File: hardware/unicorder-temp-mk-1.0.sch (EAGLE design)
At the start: 13 parts, among them IC1 TINY85

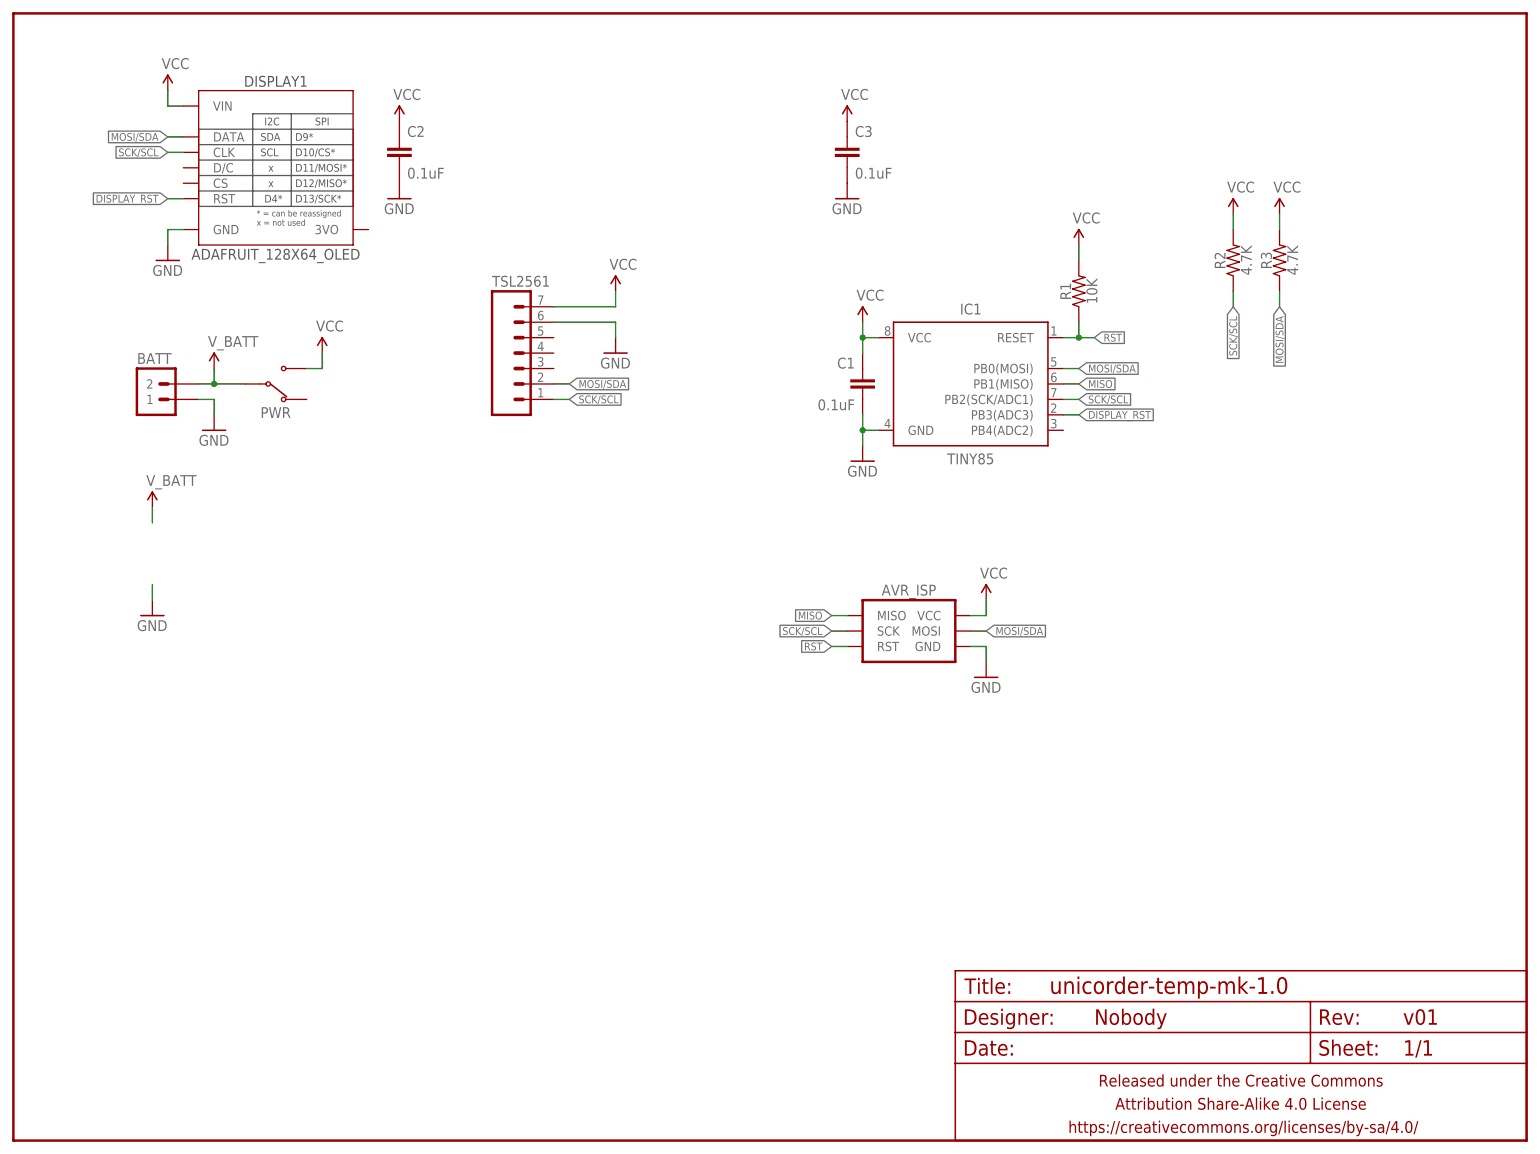
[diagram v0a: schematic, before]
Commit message: alsdkfjkalsdf
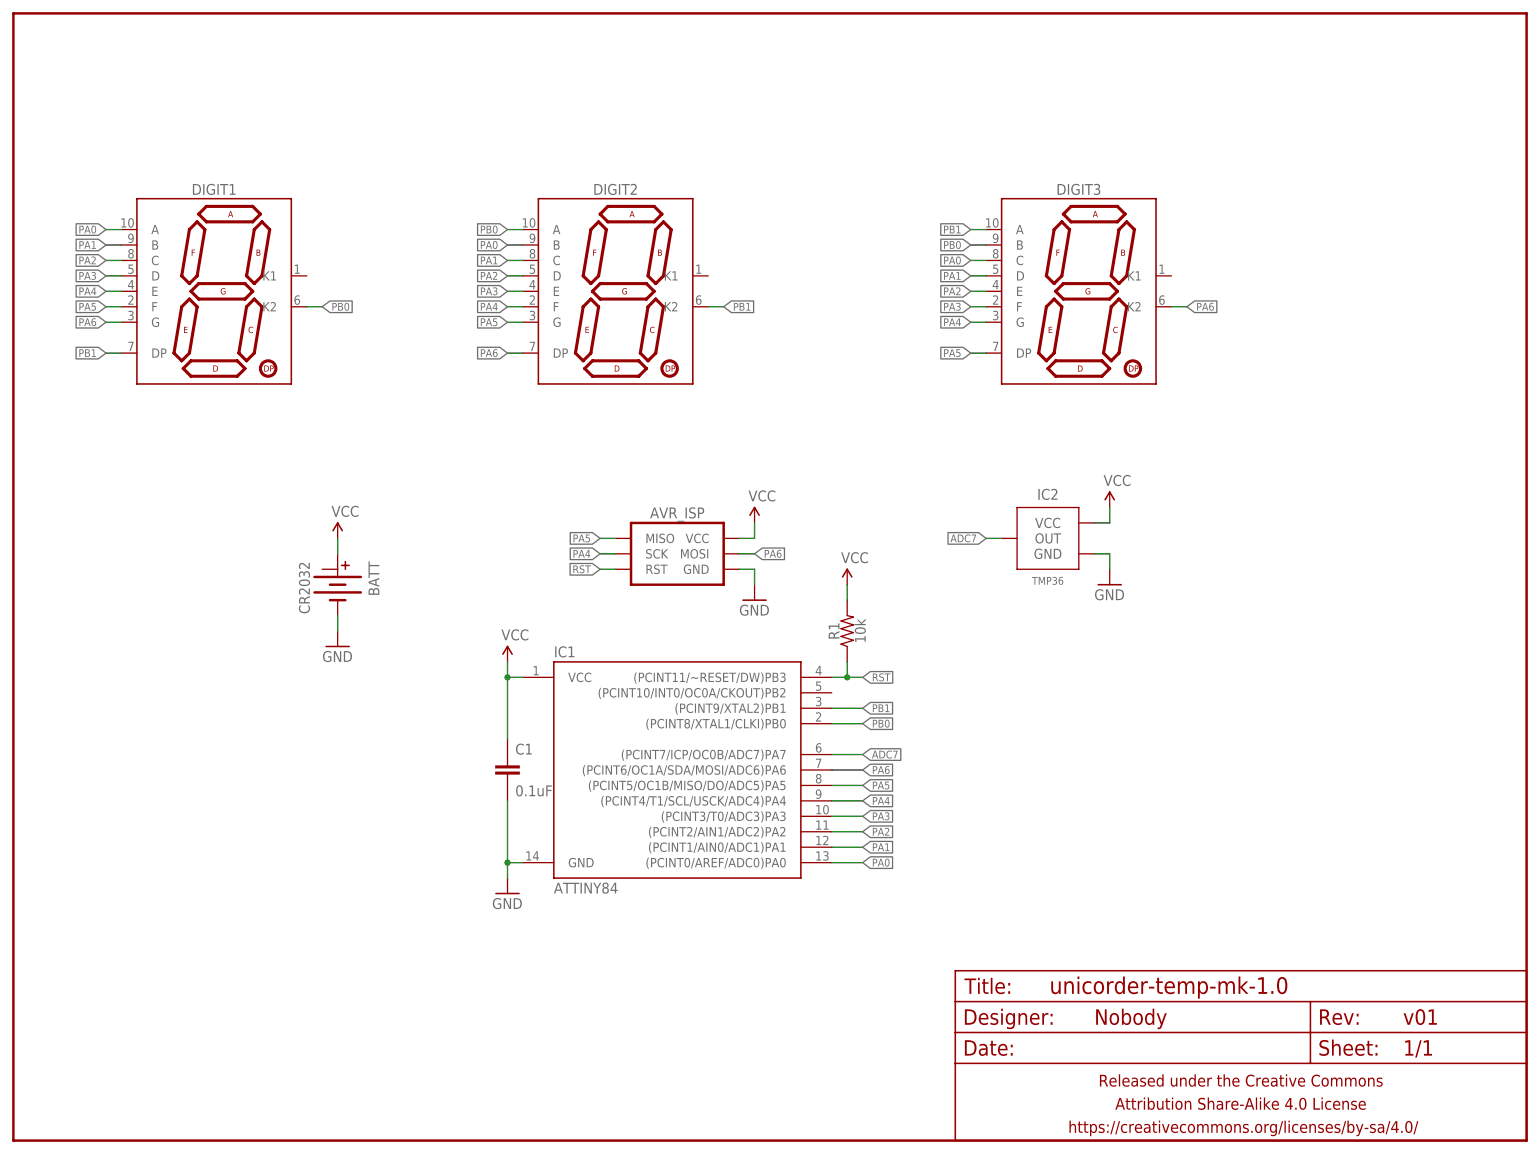
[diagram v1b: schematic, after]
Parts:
- removed C2, C3: 0.1uF, A_butts:CAPACITOR-CERAMIC025-024X044
- removed DISPLAY1: ADAFRUIT_128X64_OLED, A_butts:ADAFRUIT_128X64_OLED
- removed PWR: SWITCH-SPDTPTH-RA-2MM, A_butts:SWITCH-SPDTPTH-RA-2MM
- removed R2, R3: 4.7K, A_butts:RESISTORPTH-AXIAL-7.62MM
- removed TSL2561: (no value), A_butts:M07PTH-SLIMASS
- added DIGIT1, DIGIT2, DIGIT3: 7SEG_1DIGPTH-10MM, A_butts:7SEG_1DIGPTH-10MM
- added IC2: TMP36, A_butts:TMP36TO-92
- AVR_ISP: value AVR_SPI_PRG_6AVR-JST-PTH-RA-I2C -> AVR_SPI_PRG_6PTH; device A_butts:AVR_SPI_PRG_6AVR-JST-PTH-RA-I2C -> A_butts:AVR_SPI_PRG_6PTH
- BATT: value M02JST-PTH-VERT -> CR2032; device A_butts:M02JST-PTH-VERT -> A_butts:BATTERY-COINCR2032_SMD
- IC1: value TINY85 -> ATTINY84; device A_butts:ATTINY45TINY85-20-DIP -> A_butts:ATTINY84ATTINY84-20PU
- R1: value 10K -> 10k
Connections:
- removed net DISPLAY_RST: DISPLAY1.RST, IC1.PB3(ADC3)
- removed net MISO: AVR_ISP.MISO, IC1.PB1(MISO)
- removed net MOSI/SDA: AVR_ISP.MOSI, DISPLAY1.DATA, IC1.PB0(MOSI), R3.1, TSL2561.2
- removed net SCK/SCL: AVR_ISP.SCK, DISPLAY1.CLK, IC1.PB2(SCK/ADC1), R2.1, TSL2561.1
- removed net V_BATT: BATT.2, PWR.COM
- new net ADC7: IC1.(PCINT7/ICP/OC0B/ADC7)PA7, IC2.OUT
- new net PA0: DIGIT1.A, DIGIT2.B, DIGIT3.C, IC1.(PCINT0/AREF/ADC0)PA0
- new net PA1: DIGIT1.B, DIGIT2.C, DIGIT3.D, IC1.(PCINT1/AIN0/ADC1)PA1
- new net PA2: DIGIT1.C, DIGIT2.D, DIGIT3.E, IC1.(PCINT2/AIN1/ADC2)PA2
- new net PA3: DIGIT1.D, DIGIT2.E, DIGIT3.F, IC1.(PCINT3/T0/ADC3)PA3
- new net PA4: AVR_ISP.SCK, DIGIT1.E, DIGIT2.F, DIGIT3.G, IC1.(PCINT4/T1/SCL/USCK/ADC4)PA4
- new net PA5: AVR_ISP.MISO, DIGIT1.F, DIGIT2.G, DIGIT3.DP, IC1.(PCINT5/OC1B/MISO/DO/ADC5)PA5
- new net PA6: AVR_ISP.MOSI, DIGIT1.G, DIGIT2.DP, DIGIT3.K2, IC1.(PCINT6/OC1A/SDA/MOSI/ADC6)PA6
- new net PB0: DIGIT1.K2, DIGIT2.A, DIGIT3.B, IC1.(PCINT8/XTAL1/CLKI)PB0
- new net PB1: DIGIT1.DP, DIGIT2.K2, DIGIT3.A, IC1.(PCINT9/XTAL2)PB1
- net GND: now also BATT.-, IC2.GND; no longer BATT.1, C2.2, C3.2, DISPLAY1.GND, TSL2561.6
- net RST: now also IC1.(PCINT11/~RESET/DW)PB3; no longer IC1.RESET
- net VCC: now also BATT.+, IC2.VCC; no longer C2.1, C3.1, DISPLAY1.VIN, PWR.NO, R2.2, R3.2, TSL2561.7
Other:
- moved on the sheet: AVR_ISP, BATT, C1, R1
